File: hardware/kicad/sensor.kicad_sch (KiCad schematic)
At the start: 12 parts, among them Q4 PMV32UP, Q5 DMG1012UW, U7 BME688

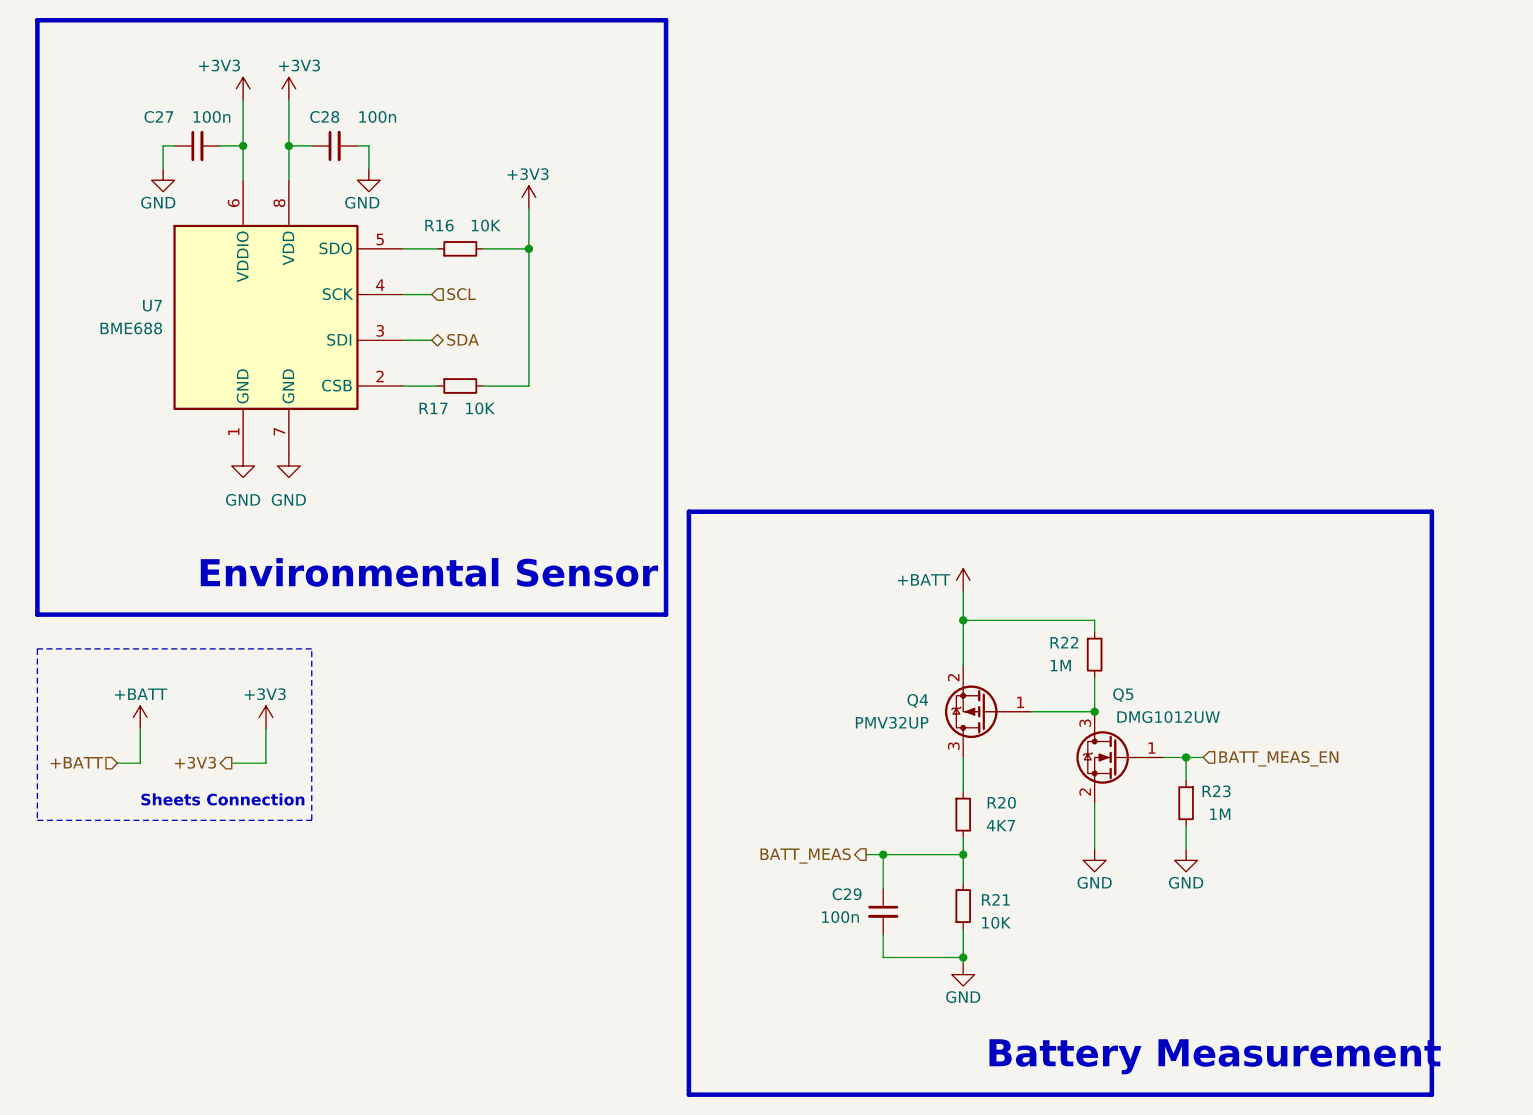
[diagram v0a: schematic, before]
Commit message: clean-up
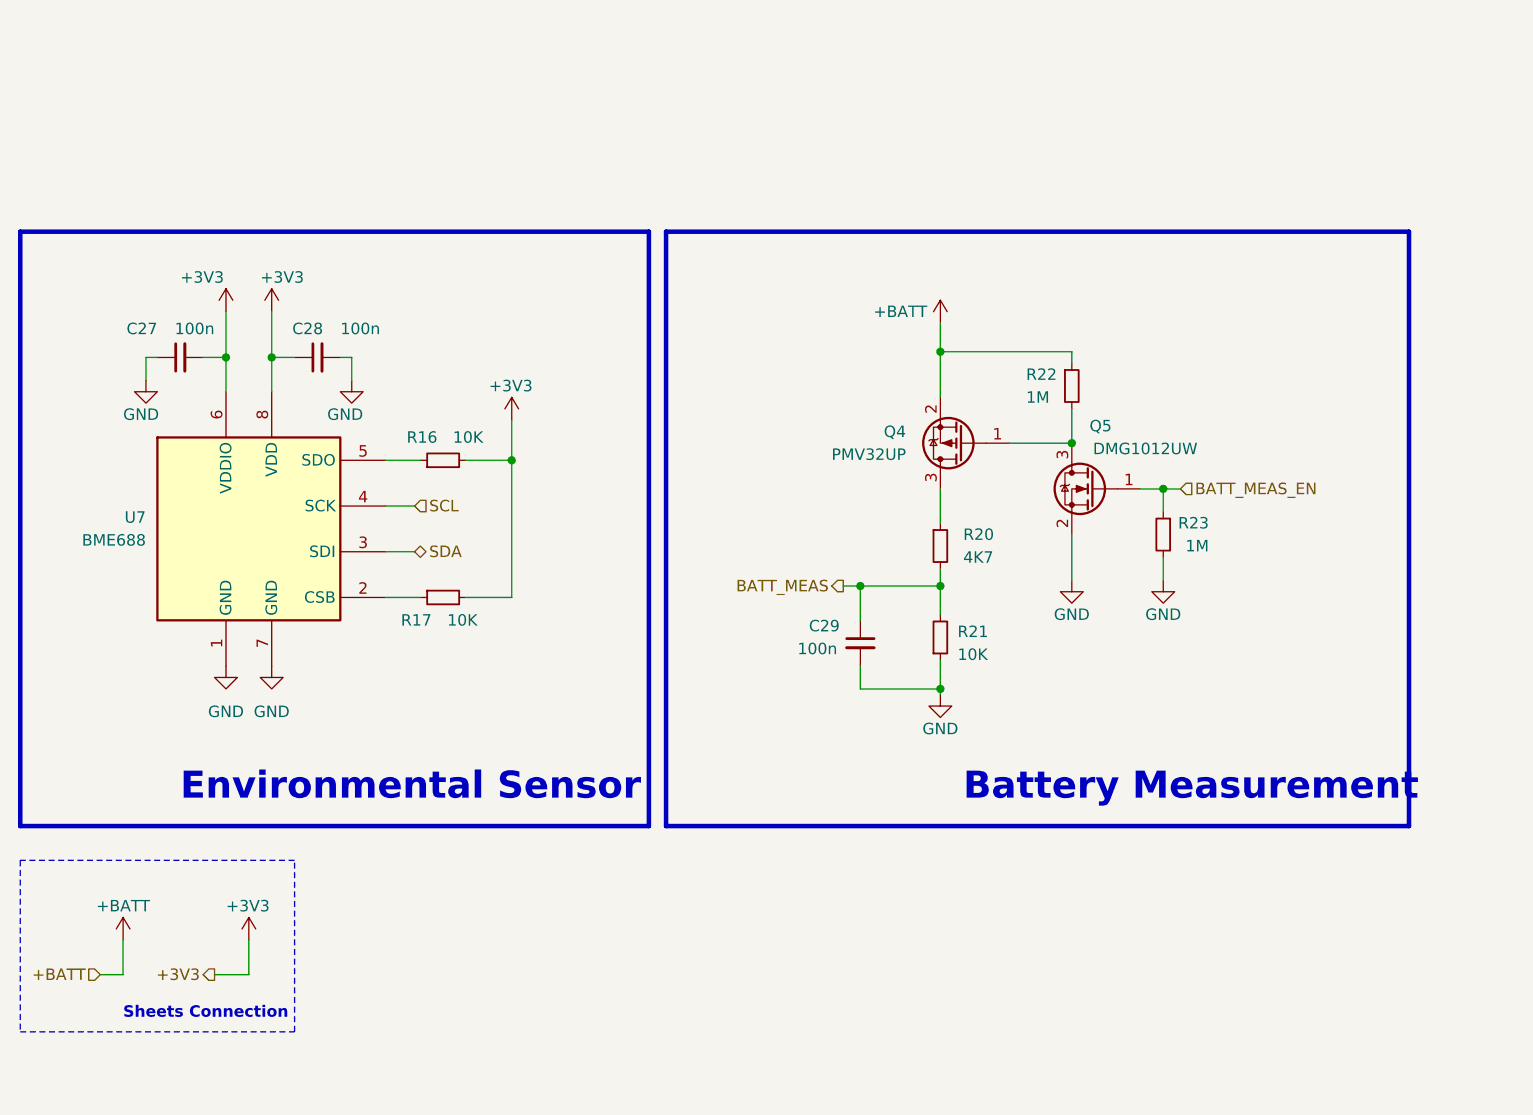
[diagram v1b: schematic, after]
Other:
- moved on the sheet: C27, C28, C29, Q4, Q5, R16, R17, R20, R21, R22, R23, U7
